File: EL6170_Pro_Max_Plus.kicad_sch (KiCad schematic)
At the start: 176 parts, among them CN1 PJ-327A0-SMT, J1 USB_C_Receptacle, J2 microSD, Q1 MMBT3904, Q2 MMBT3904, Q3 2N7002, Q4 AO3401A, Q5 AO3401A, SW1 SW_LEFT, SW10 SW_K4, SW11 SW_K5, SW12 SW_K6, SW13 SW_K7, SW14 SW_K8, SW15 SW_K9, SW16 SW_K0, SW17 SW_KQ, SW18 SW_KW, SW19 SW_KE, SW2 SW_UP, SW20 SW_KR, SW21 SW_KT, SW22 SW_KY, SW23 SW_KU, SW24 SW_KI, SW25 SW_KO, SW26 SW_KP, SW27 SW_KA, SW28 SW_KS, SW29 SW_KD, SW3 SW_DOWN, SW30 SW_KF, SW31 SW_KG, SW32 SW_KH, SW33 SW_KJ, SW34 SW_KK, SW35 SW_KL, SW36 SW_KZ, SW37 SW_KX, SW38 SW_KC, SW39 SW_KV, SW4 SW_RIGHT, SW40 SW_KB, SW41 SW_KN, SW42 SW_KM, SW43 SW_KCOM, SW44 SW_KDOT, SW45 SW_SHIFT, SW46 SW_CE(IO0), SW47 SW_OFF, SW48 SW_SECRET, SW49 SW_MCK, SW5 SW_UP2, SW50 SW_SPACE, SW51 SW_REMARK, SW52 SW_CALENDAR, SW53 SW_MODE, SW54 SW_ENTER, SW6 SW_DOWN2, SW7 SW_K1, SW8 SW_K2, SW9 SW_K3, U1 ESP32-S3, U10 ME6211C33M5, U11 TP5400_C2891434, U12 PCF8575DBR, U2 TPS61040DBV, U3 ESP-PSRAM64H, U4 W25Q128JVS, U5 ME6217C33M5, U6 CH340K, U7 RFANT5220110A0T, U8 CH334R, U9 PCM5102A, X1 40MHz, X2 12MHz

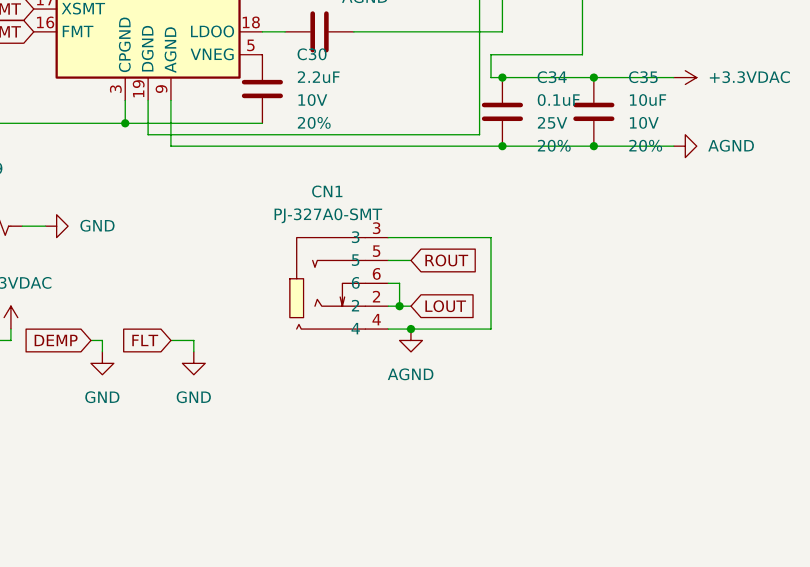
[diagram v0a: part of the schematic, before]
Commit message: PCM5102A
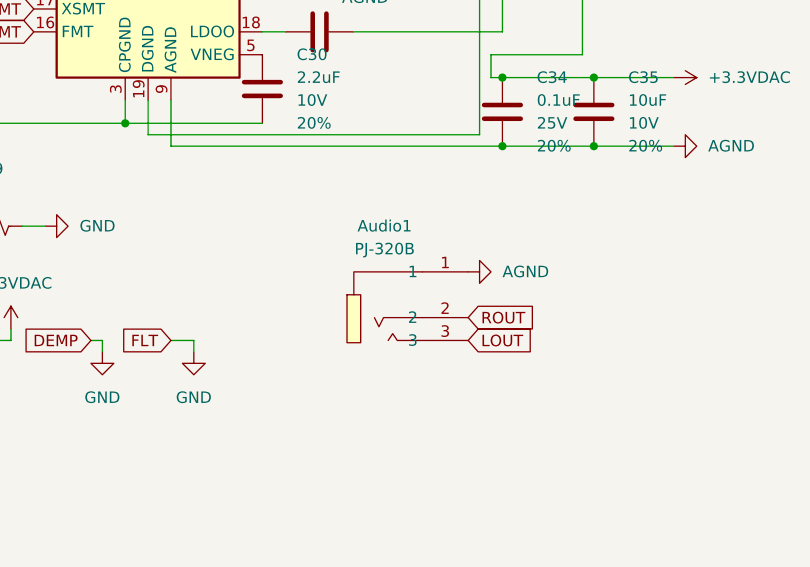
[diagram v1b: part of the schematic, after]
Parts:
- removed CN1: PJ-327A0-SMT, easyeda2kicad:AUDIO-SMD_PJ-327A0-SMT, symbol easyeda2kicad:PJ-327A0-SMT
- added Audio1: PJ-320B, easyeda2kicad:AUDIO-SMD_PJ-320B, symbol easyeda2kicad:PJ-320B
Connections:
- net AGND: now also Audio1.1
- net LOUT: now also Audio1.3
- net ROUT: now also Audio1.2
